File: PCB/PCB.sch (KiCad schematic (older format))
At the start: 40 parts, among them J1 Dynamo, J10 Conn_01x08_Female, J11 Conn_01x01_Female, J12 Conn_01x04_Female, J2 Conn_01x28_Female, J3 Conn_01x02_Female, J4 Conn_01x02_Female, J5 Conn_01x02_Female, J6 Conn_01x02_Female, J7 Conn_01x08_Female, J8 Conn_01x02_Female, J9 Conn_01x03_Female, U1 BA33BC0T, Y1 16MHz

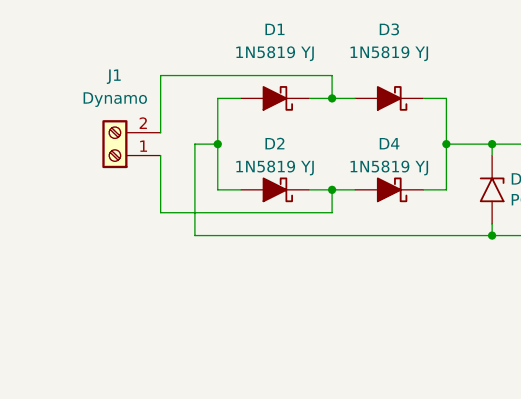
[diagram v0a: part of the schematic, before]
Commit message: Added PCB images
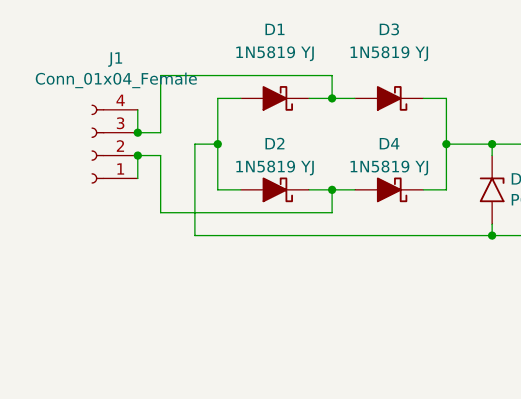
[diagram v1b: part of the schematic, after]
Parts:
- removed J1: Dynamo, TerminalBlock:TerminalBlock_Altech_AK300-2_P5.00mm, symbol Connector:Screw_Terminal_01x02
- added J1: Conn_01x04_Female, Connector_Molex:Molex_KK-396_A-41791-0004_1x04_P3.96mm_Vertical, symbol Connector:Conn_01x04_Female
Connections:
- net at D2.1 (K), D4.2 (A): now also J1.1 (Pin_1), J1.2 (Pin_2)
- net at D1.1 (K), D3.2 (A): now also J1.3 (Pin_3), J1.4 (Pin_4)
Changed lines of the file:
@@
 EESchema Schematic File Version 4
 LIBS:PCB-cache
-EELAYER 29 0
+EELAYER 26 0
 EELAYER END
 $Descr A4 11693 8268
@@
 	-1   0    0    1
 $EndComp
-$Comp
-L Connector:Screw_Terminal_01x02 J1
-U 1 1 5E63414E
-P 1550 1300
-F 0 "J1" H 1550 950 50  0000 C CNN
-F 1 "Dynamo" H 1550 1050 50  0000 C CNN
-F 2 "TerminalBlock:TerminalBlock_Altech_AK300-2_P5.00mm" H 1550 1300 50  0001 C CNN
-F 3 "~" H 1550 1300 50  0001 C CNN
-	1    1550 1300
-	-1   0    0    1
-$EndComp
 Wire Wire Line
 	2100 1050 2000 1050
@@
 NoConn ~ 2850 4450
 NoConn ~ 2850 4550
+$Comp
+L Connector:Conn_01x04_Female J1
+U 1 1 5E2F9CB0
+P 1450 1300
+F 0 "J1" H 1344 875 50  0000 C CNN
+F 1 "Conn_01x04_Female" H 1344 966 50  0000 C CNN
+F 2 "Connector_Molex:Molex_KK-396_A-41791-0004_1x04_P3.96mm_Vertical" H 1450 1300 50  0001 C CNN
+F 3 "~" H 1450 1300 50  0001 C CNN
+	1    1450 1300
+	-1   0    0    1
+$EndComp
+Wire Wire Line
+	1750 1200 1650 1200
+Wire Wire Line
+	1750 1300 1650 1300
+Wire Wire Line
+	1650 1200 1650 1100
+Connection ~ 1650 1200
+Wire Wire Line
+	1650 1300 1650 1400
+Connection ~ 1650 1300
 $EndSCHEMATC
